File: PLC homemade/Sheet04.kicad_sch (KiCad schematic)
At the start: 0 parts

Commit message: :spanner:At interfaces
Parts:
- added C29: 100nF 50V, symbol Device:C
- added R36, R37, R38, R39, R40, R41: 4K7, symbol Device:R
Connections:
- new net 3V3: C29.1
- new net GND: C29.2

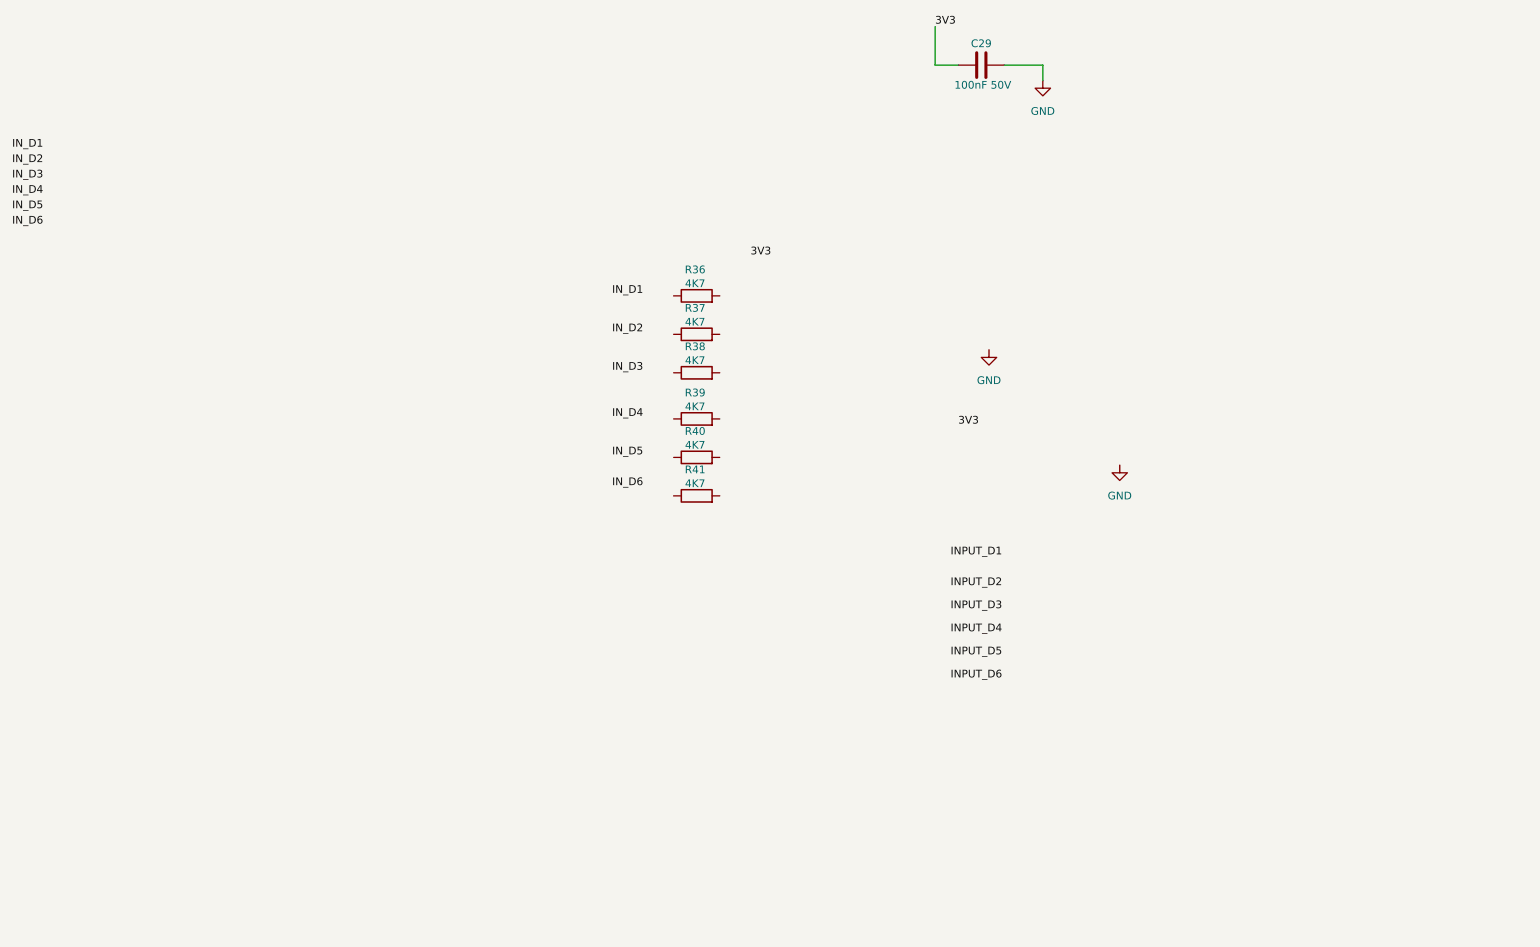
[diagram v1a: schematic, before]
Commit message: :rocket: started on OUTPUT
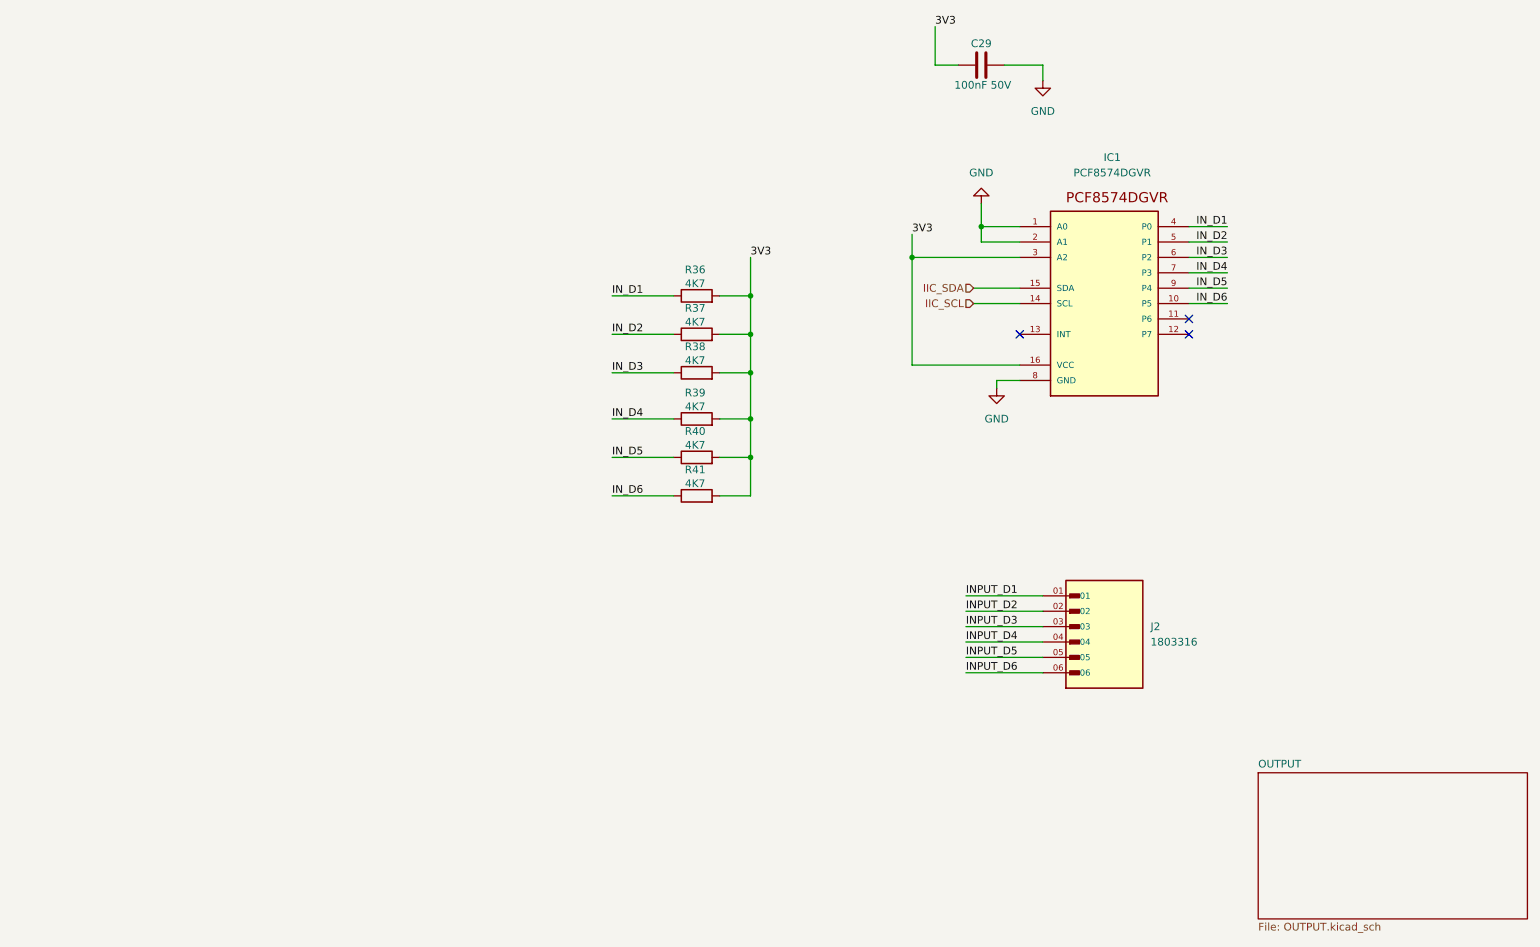
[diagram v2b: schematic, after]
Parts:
- added IC1: PCF8574DGVR, PCF8574DGVR:DIL16, symbol PCF8574DGVR:PCF8574DGVR
- added J2: 1803316, 1803316:PHOENIX_1803316, symbol 1803316:1803316
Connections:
- net 3V3: now also R36.2, R37.2, R38.2, R39.2, R40.2, R41.2, IC1.16 (VCC), IC1.3 (A2)
- net GND: now also IC1.1 (A0), IC1.2 (A1), IC1.8 (GND)
- net INPUT_D1: now also J2.01
- net INPUT_D2: now also J2.02
- net INPUT_D3: now also J2.03
- net INPUT_D4: now also J2.04
- net INPUT_D5: now also J2.05
- net INPUT_D6: now also J2.06
- net IN_D1: now also R36.1, IC1.4 (P0)
- net IN_D2: now also R37.1, IC1.5 (P1)
- net IN_D3: now also R38.1, IC1.6 (P2)
- net IN_D4: now also R39.1, IC1.7 (P3)
- net IN_D5: now also R40.1, IC1.9 (P4)
- net IN_D6: now also R41.1, IC1.10 (P5)
- new net IIC_SCL: IC1.14 (SCL)
- new net IIC_SDA: IC1.15 (SDA)
- no-connect marks 0 -> 3
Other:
- added sheet OUTPUT (OUTPUT.kicad_sch)
